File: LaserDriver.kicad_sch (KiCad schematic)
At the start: 30 parts, among them J100 Screw_Terminal_01x04, J101 Screw_Terminal_01x02, J102 nano_left, J103 nano_right, U100 TPS92513DGQR

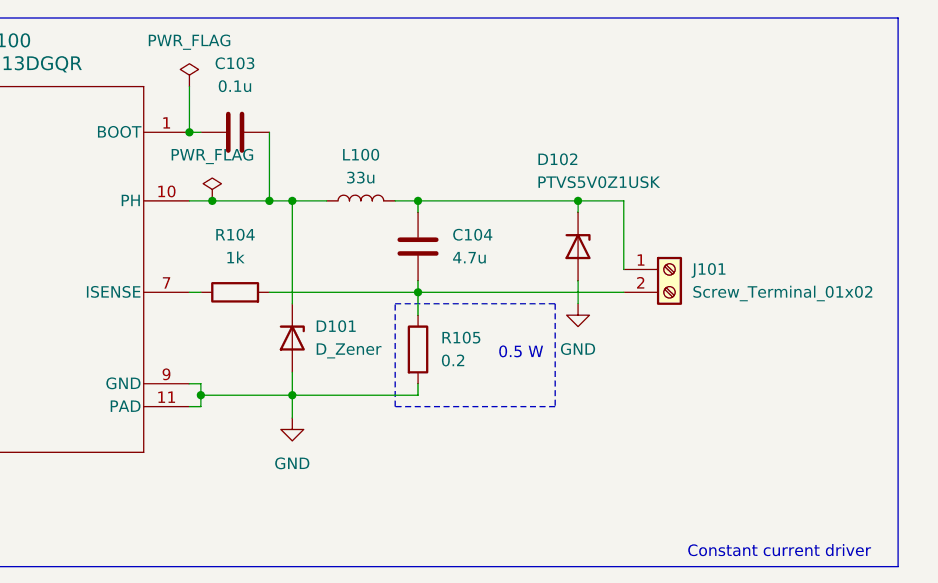
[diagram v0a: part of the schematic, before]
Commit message: fixed errors
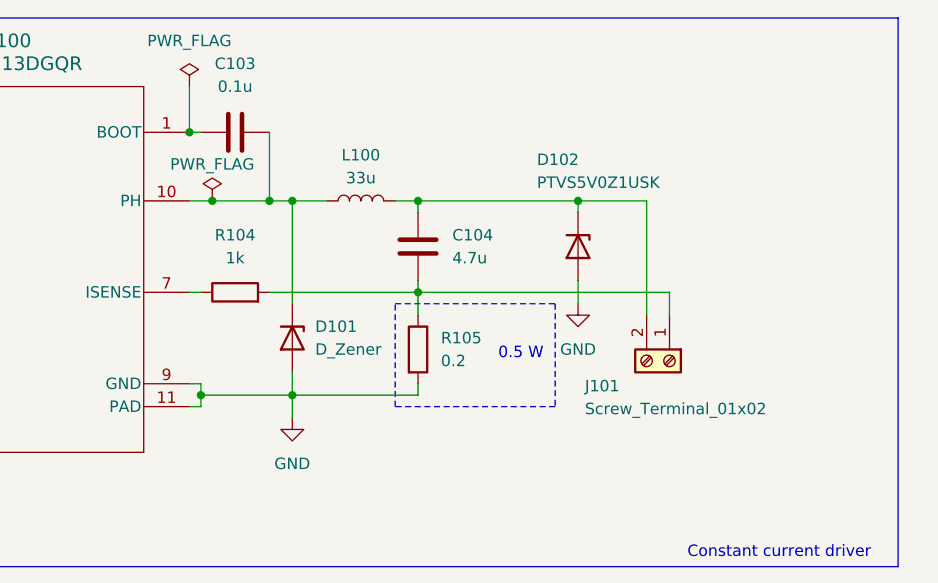
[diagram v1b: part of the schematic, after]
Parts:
- U100: footprint TPS:DGQ0010D_L -> TPS:DGQ0010D_NV_L
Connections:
- net at C104.1, D102.1 (K), L100.2: now also J101.2 (Pin_2); no longer J101.1 (Pin_1)
- net at C104.2, R104.2, R105.1: now also J101.1 (Pin_1); no longer J101.2 (Pin_2)
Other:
- moved on the sheet: J101
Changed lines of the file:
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@@
 	(wire
 		(pts
+			(xy 173.99 49.53) (xy 173.99 52.07)
+		)
+		(stroke
+			(width 0)
+			(type default)
+		)
+	)
+	(wire
+		(pts
 			(xy 33.02 120.65) (xy 36.83 120.65)
 		)
@@
 	(wire
 		(pts
-			(xy 163.83 39.37) (xy 168.91 39.37)
+			(xy 163.83 39.37) (xy 171.45 39.37)
 		)
 		(stroke
@@
 	(wire
 		(pts
-			(xy 168.91 39.37) (xy 168.91 46.99)
+			(xy 171.45 39.37) (xy 171.45 52.07)
 		)
 		(stroke
@@
 	(wire
 		(pts
-			(xy 146.05 49.53) (xy 168.91 49.53)
+			(xy 146.05 49.53) (xy 173.99 49.53)
 		)
 		(stroke
@@
 	(symbol
 		(lib_id "Connector:Screw_Terminal_01x02")
-		(at 173.99 46.99 0)
+		(at 173.99 57.15 270)
 		(unit 1)
 		(exclude_from_sim no)
@@
 		(on_board yes)
 		(dnp no)
-		(fields_autoplaced yes)
 		(property "Reference" "J101"
-			(at 176.53 46.9899 0)
+			(at 164.592 59.944 90)
 			(effects
 				(font
@@
 		)
 		(property "Value" "Screw_Terminal_01x02"
-			(at 176.53 49.5299 0)
+			(at 164.592 62.484 90)
 			(effects
 				(font
@@
 		)
 		(property "Footprint" "TerminalBlock:TerminalBlock_Xinya_XY308-2.54-2P_1x02_P2.54mm_Horizontal"
-			(at 173.99 46.99 0)
+			(at 173.99 57.15 0)
 			(effects
 				(font
@@
 		)
 		(property "Datasheet" "~"
-			(at 173.99 46.99 0)
+			(at 173.99 57.15 0)
 			(effects
 				(font
@@
 		)
 		(property "Description" "Generic screw terminal, single row, 01x02, script generated (kicad-library-utils/schlib/autogen/connector/)"
-			(at 173.99 46.99 0)
+			(at 173.99 57.15 0)
 			(effects
 				(font
@@
 		(on_board yes)
 		(dnp no)
-		(fields_autoplaced yes)
 		(property "Reference" "#FLG02"
 			(at 123.19 37.465 0)
@@
 		)
 		(property "Value" "PWR_FLAG"
-			(at 123.19 34.29 0)
+			(at 123.19 35.306 0)
 			(effects
 				(font
@@
 			)
 		)
-		(property "Footprint" "TPS:DGQ0010D_L"
+		(property "Footprint" "TPS:DGQ0010D_NV_L"
 			(at 100.33 46.99 0)
 			(effects
